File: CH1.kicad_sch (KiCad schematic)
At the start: 27 parts, among them IC201 TS12A4516DBVR, J101 CH1, SW101 AC/DC, U102 OPA356xxDBV, U104 OPA356xxDBV, U203 TLP176AM

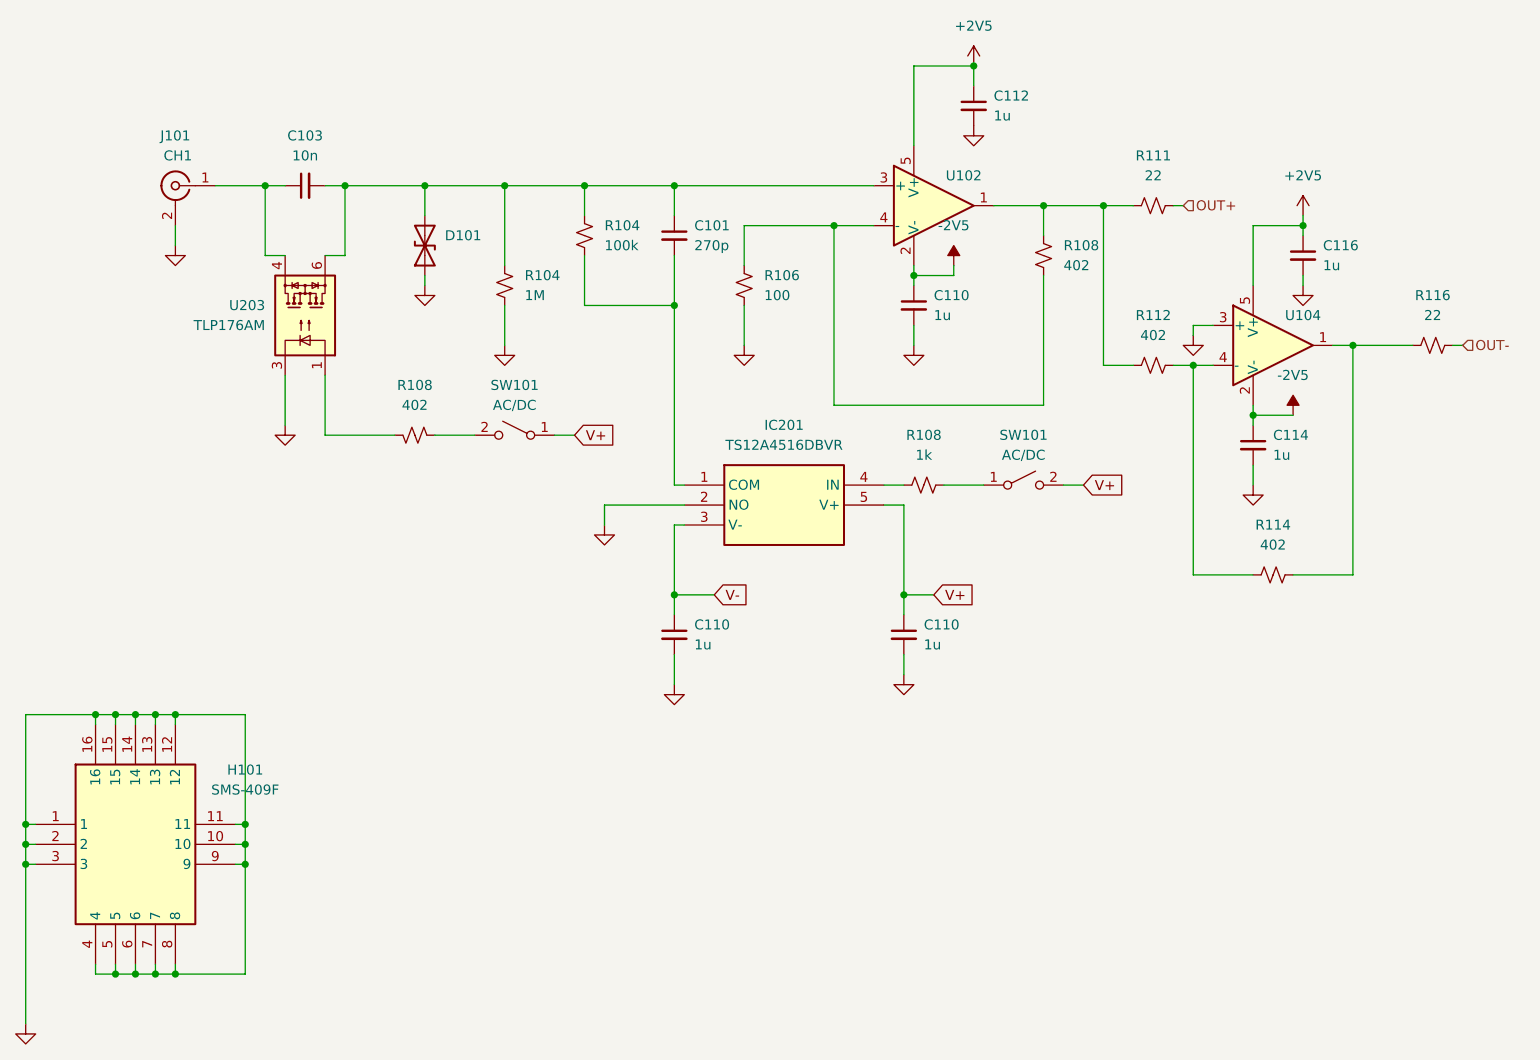
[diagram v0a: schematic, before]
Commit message: v3 done
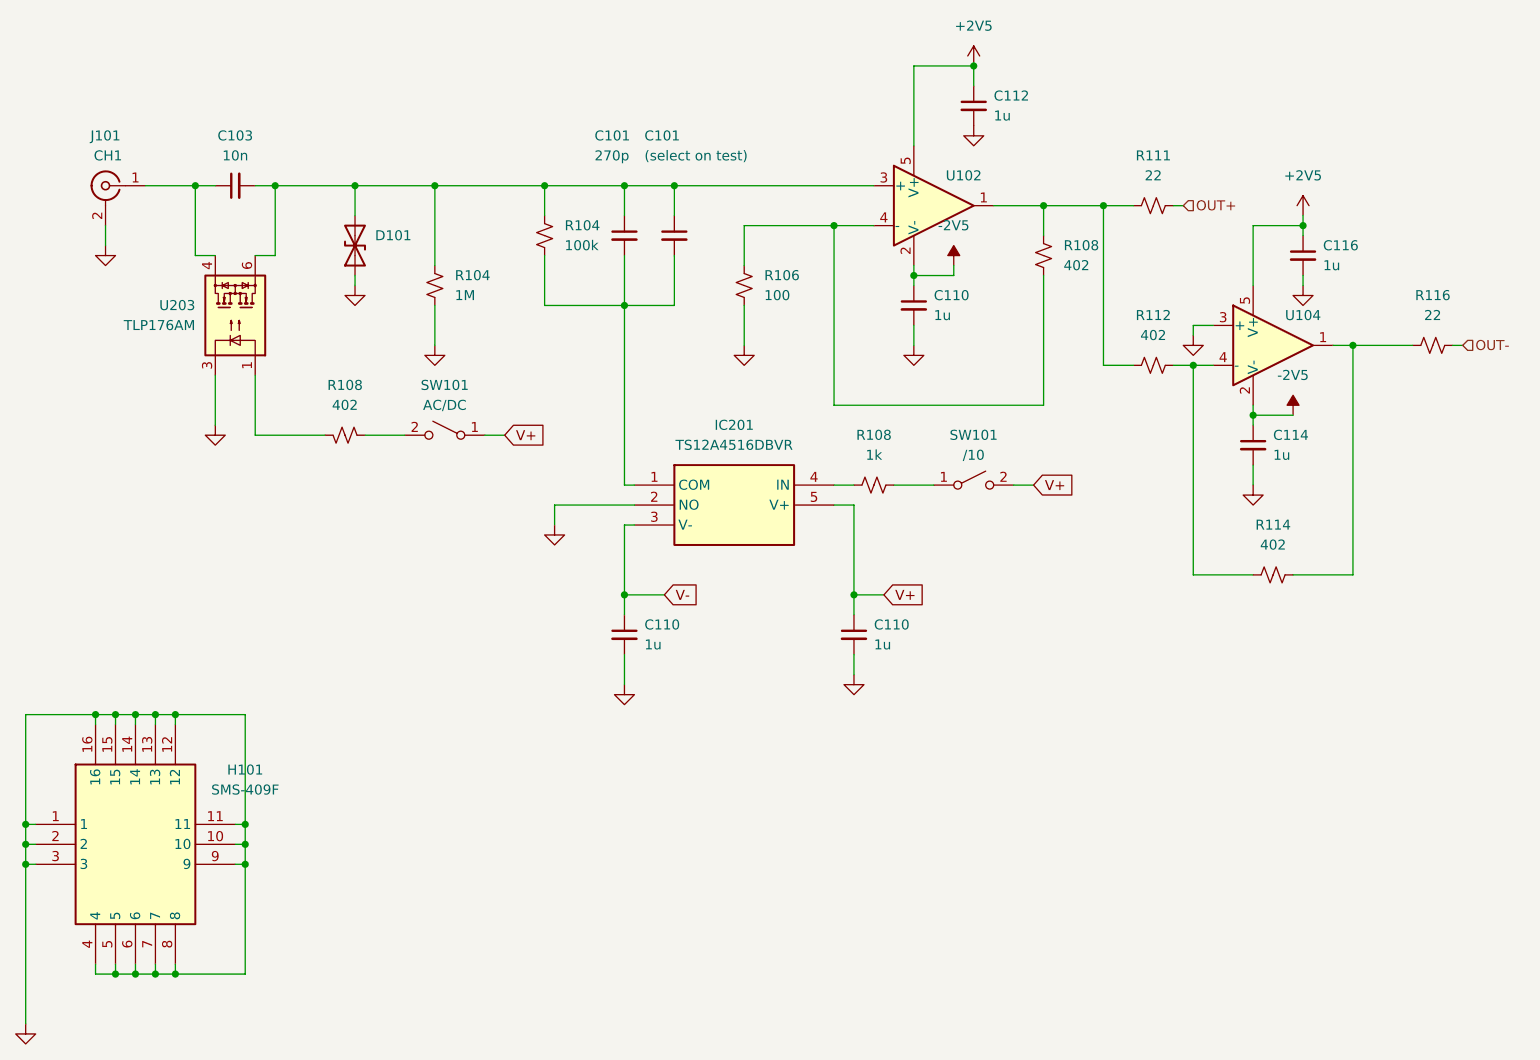
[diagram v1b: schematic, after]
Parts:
- added C101: (select on test), Capacitor_SMD:C_0402_1005Metric_Pad0.74x0.62mm_HandSolder, symbol Device:C_Small
- SW101: value AC/DC -> /10
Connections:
- net at C101.1, C103.2, D101.2 (A2)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: now also C101.1
- net at C101.2, IC201.1 (COM), R104.2: now also C101.2
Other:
- moved on the sheet: C101, C103, C110, D101, IC201, J101, R104, R108, SW101, U203
